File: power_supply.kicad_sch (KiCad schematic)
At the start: 27 parts, among them J1 Conn_01x02, J2 Conn_01x02, U3 L78L09_SOT89, U4 LM4040DBZ-2.0, U5 L78L09_SOT89

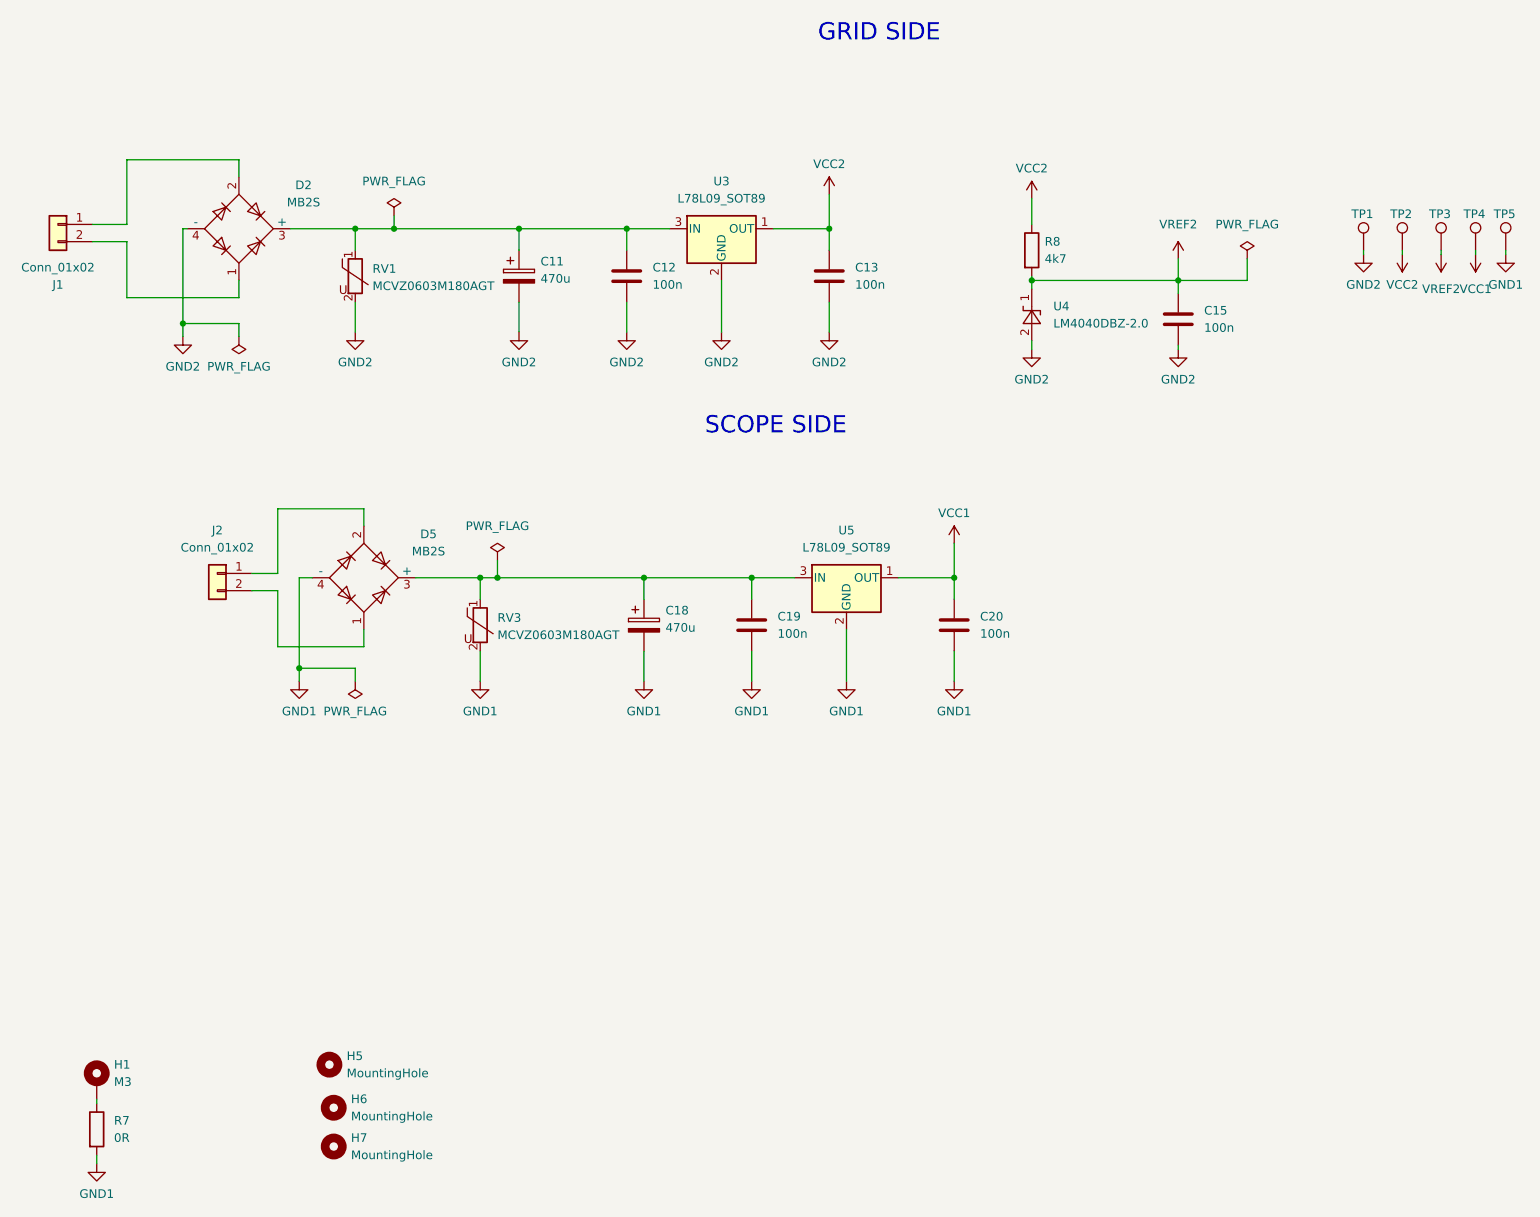
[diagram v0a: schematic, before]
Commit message: Redesign pcb
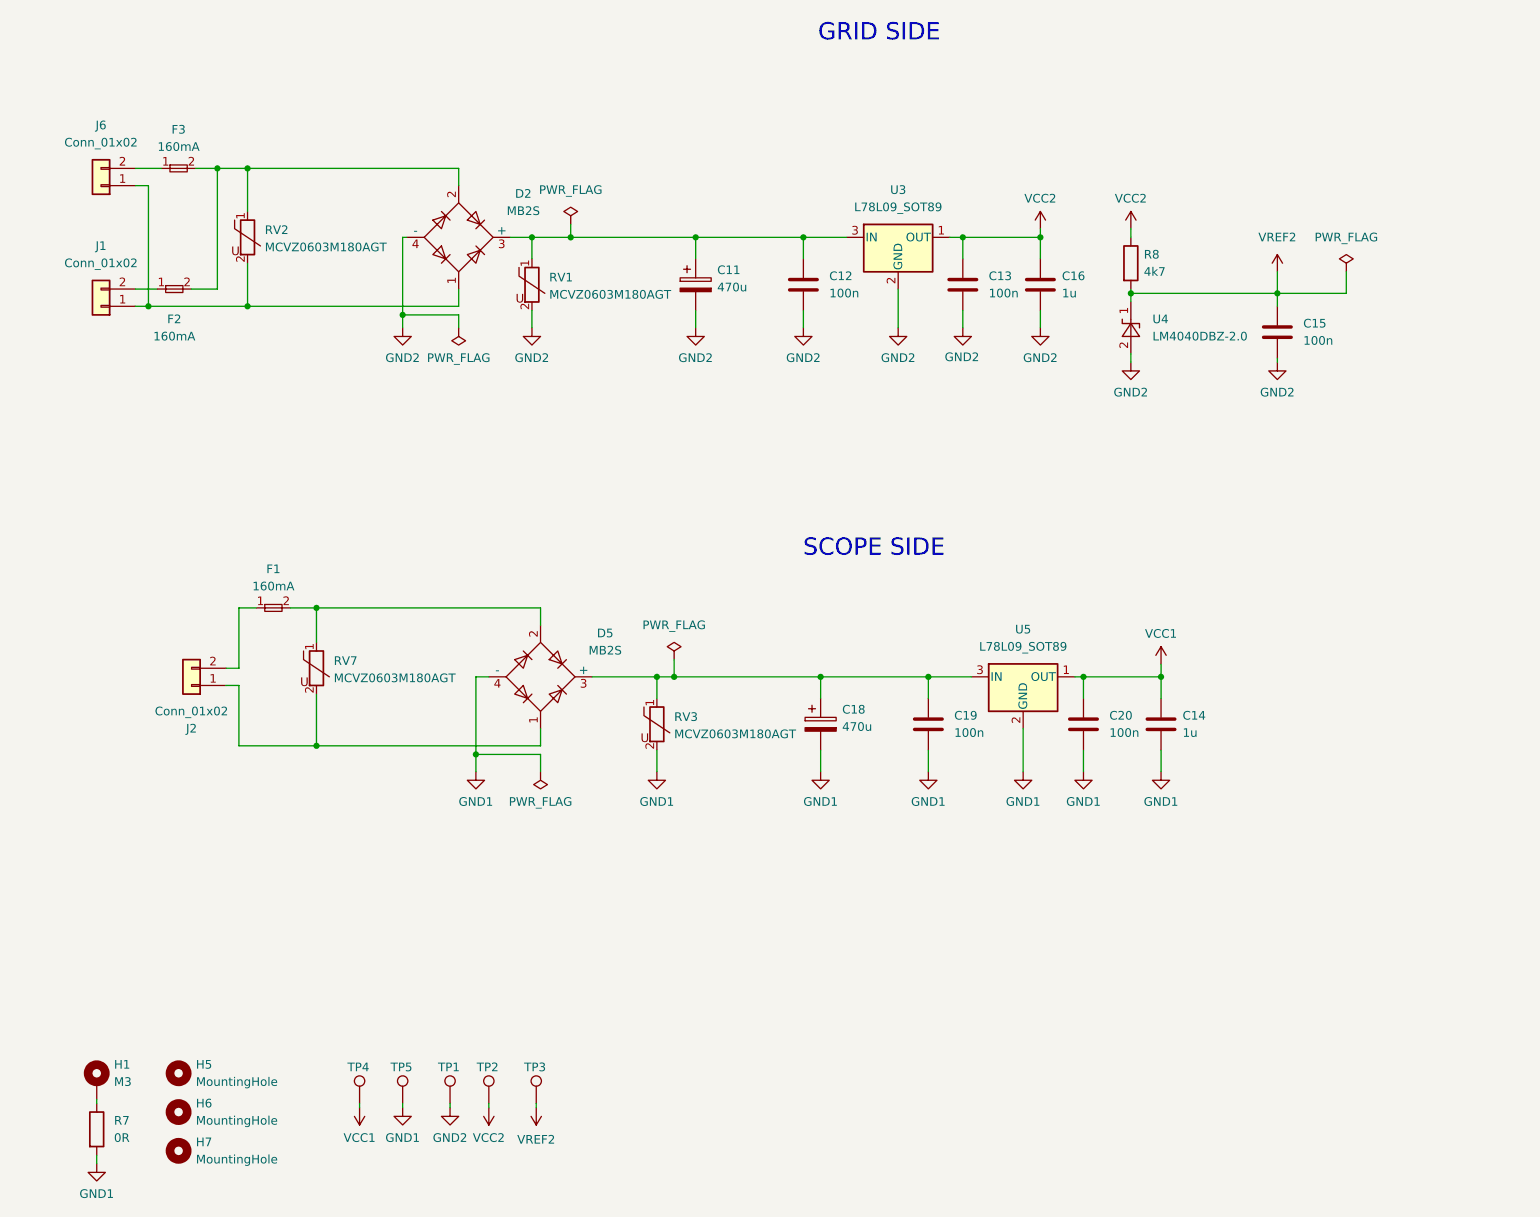
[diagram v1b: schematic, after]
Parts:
- added C14, C16: 1u, Capacitor_SMD:C_0603_1608Metric, symbol Koszalix_Capacitors_Ceramic_Walsin_0603:CAP_1u_X7R
- added F1, F2, F3: 160mA, Fuse:Fuse_1206_3216Metric_Pad1.42x1.75mm_HandSolder, symbol Koszalix_Fuses:Polyfuse_SMD_160mA_1206
- added J6: Conn_01x02, Connector_JST:JST_XH_B2B-XH-A_1x02_P2.50mm_Vertical, symbol Connector_Generic:Conn_01x02
- added RV2, RV7: MCVZ0603M180AGT, Resistor_SMD:R_0603_1608Metric_Pad0.98x0.95mm_HandSolder, symbol Koszalix_Varistors:MCVZ0603M180AGT
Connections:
- net GND1: now also C14.2
- net GND2: now also C16.2
- net VCC1: now also C14.1
- net VCC2: now also C16.1
- net at D2.1: now also J1.1 (Pin_1), J6.1 (Pin_1), RV2.2; no longer J1.2 (Pin_2)
- net at D2.2: now also F2.2, F3.2, RV2.1; no longer J1.1 (Pin_1)
- net at J2.2 (Pin_2): now also F1.1; no longer D5.1
- net at D5.2: now also F1.2, RV7.1; no longer J2.1 (Pin_1)
- new net: F3.1, J6.2 (Pin_2)
- new net: F2.1, J1.2 (Pin_2)
- new net: D5.1, J2.1 (Pin_1), RV7.2
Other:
- moved on the sheet: C11, C12, C13, C15, C18, C19, C20, D2, D5, H5, H6, H7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
